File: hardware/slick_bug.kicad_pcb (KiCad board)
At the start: 2 copper layers, 20.2 x 40.8 mm, 8 parts, among them J1 Conn_01x04_Socket, J2 Conn_01x04_Socket, U1 XIAO-RP2040-SMD, U4 MAX40203AUK+T

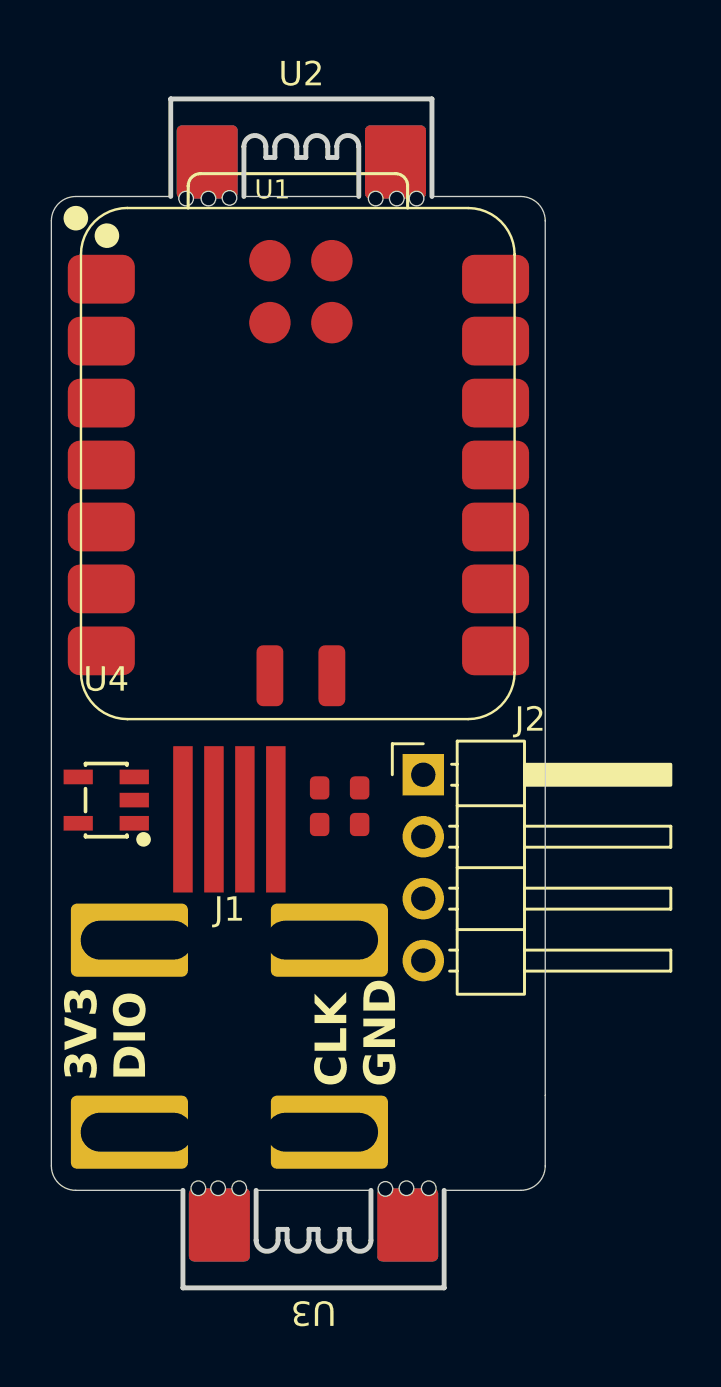
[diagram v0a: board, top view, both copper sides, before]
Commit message: tweaks
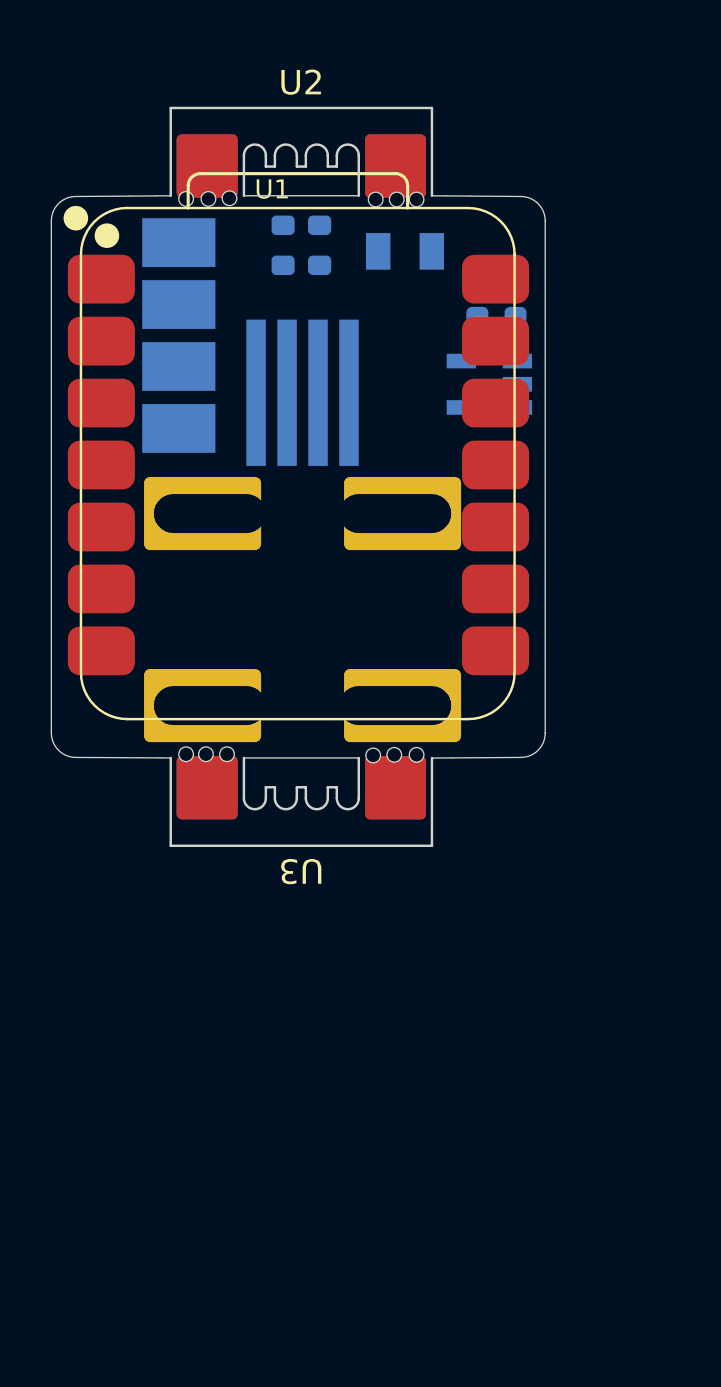
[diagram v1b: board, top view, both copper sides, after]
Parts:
- added C1: 1uF, PCM_JLCPCB:C_0603, B.Cu at (98.8, 65.0)
- added F1: JK-SMD0805-020-30V, easyeda:F0805, B.Cu at (95.0, 62.2)
- J1, R1, R2, U4: moved to B.Cu
- J2: footprint Connector_PinHeader_2.54mm:PinHeader_1x04_P2.54mm_Horizontal -> halfr:Harwin_M20-89004xx_1x04_P2.54mm_Horizontal_blank; moved to B.Cu
- moved R2 23.9 mm to (90.0, 62.0), turned to -90 degrees
- moved J2 23.8 mm to (80.2, 65.7), turned to 180 degrees
- moved U4 23.2 mm to (98.5, 67.7)
- moved R1 22.3 mm to (91.5, 62.0), turned to -90 degrees
- moved U3 18.1 mm to (90.8, 84.8)
- moved J1 17.7 mm to (90.8, 72.2), turned to 180 degrees
- moved U2 0.37 mm to (90.8, 58.2)
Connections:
- U4 pad 1: Net-(U1-3V3_OUT) -> Net-(U4-EN)
- U4 pad 3: Net-(U1-3V3_OUT) -> Net-(U4-EN)
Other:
- board size 20.2 x 40.8 mm -> 20.2 x 23.1 mm
- board text added: "IO"
- board text added: "SLICKBUG V1"
- board text removed: "DIO"
- board text removed: "Slick Bug V1"
